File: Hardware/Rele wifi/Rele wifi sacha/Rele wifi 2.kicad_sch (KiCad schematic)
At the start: 16 parts, among them J1 Screw_Terminal_01x02, J2 Screw_Terminal_01x03, J4 Conn_01x03_Pin, K1 G5LE-1, Q2 BC337, SW1 SW_Push, U5 PC817

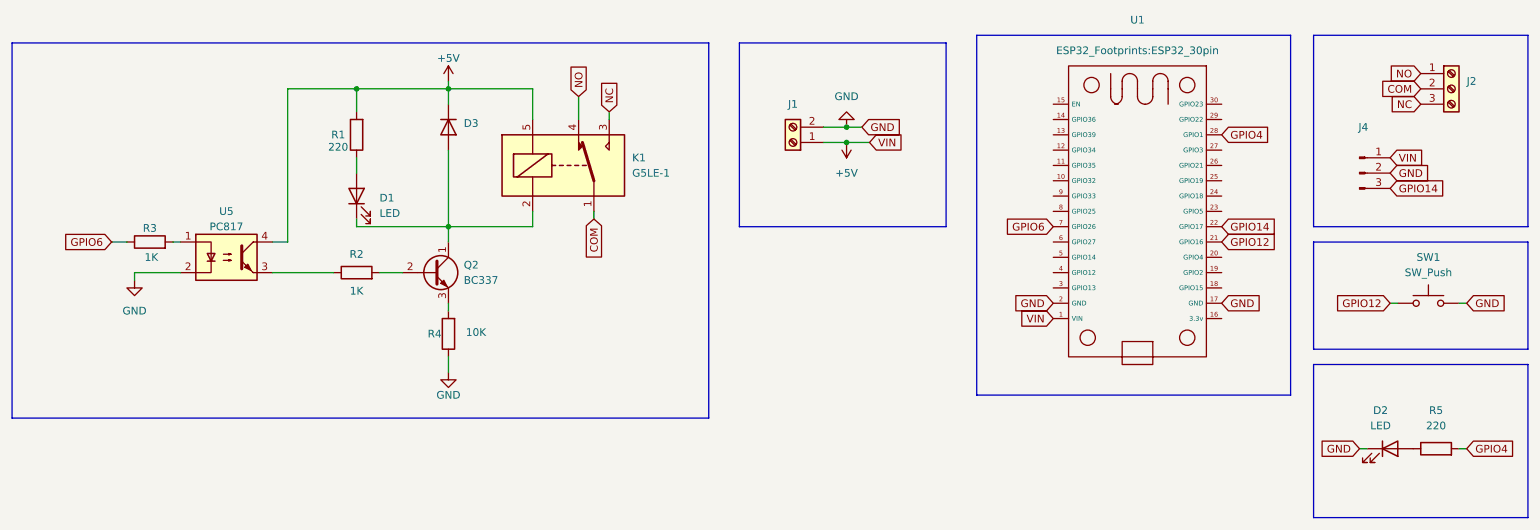
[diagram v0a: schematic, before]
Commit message: actu pcb
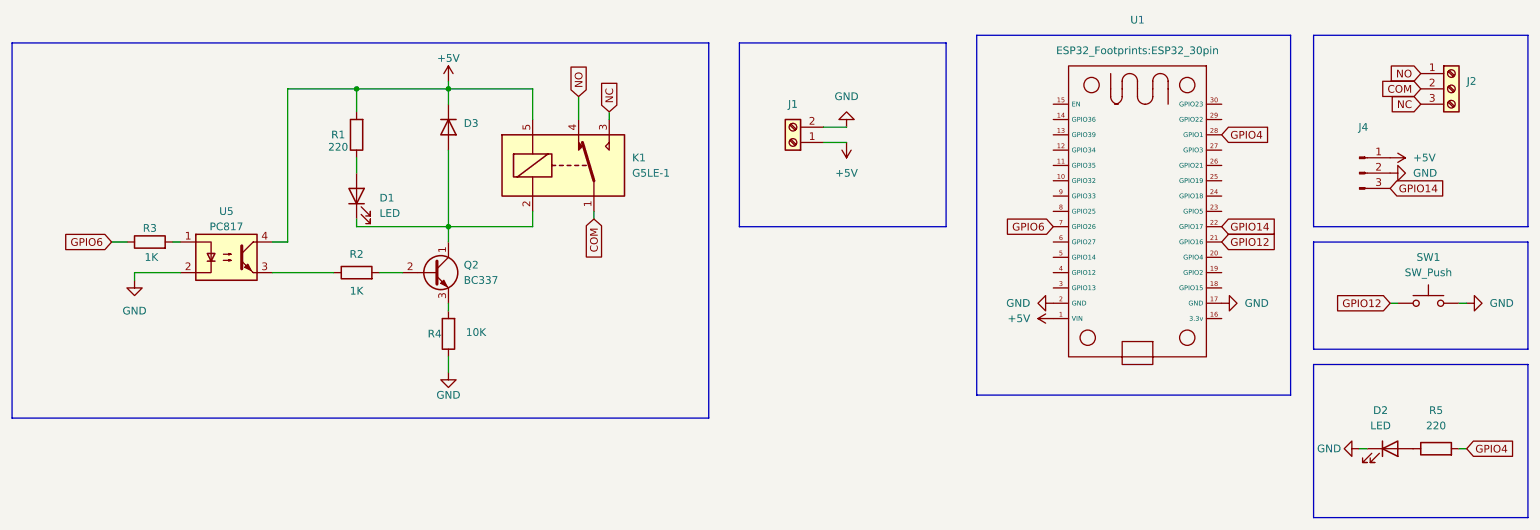
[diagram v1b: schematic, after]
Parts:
- J1: footprint TerminalBlock:TerminalBlock_MaiXu_MX126-5.0-02P_1x02_P5.00mm -> TerminalBlock_Phoenix:TerminalBlock_Phoenix_MKDS-1,5-2-5.08_1x02_P5.08mm_Horizontal
- J2: footprint TerminalBlock:TerminalBlock_MaiXu_MX126-5.0-03P_1x03_P5.00mm -> TerminalBlock_Phoenix:TerminalBlock_Phoenix_MKDS-1,5-3-5.08_1x03_P5.08mm_Horizontal
- J4: footprint Connector_PinHeader_2.00mm:PinHeader_1x03_P2.00mm_Vertical -> Connector_PinSocket_2.54mm:PinSocket_1x03_P2.54mm_Vertical

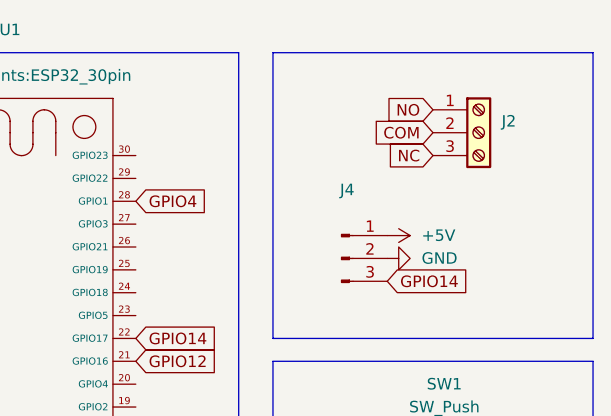
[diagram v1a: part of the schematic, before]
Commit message: actu pcb
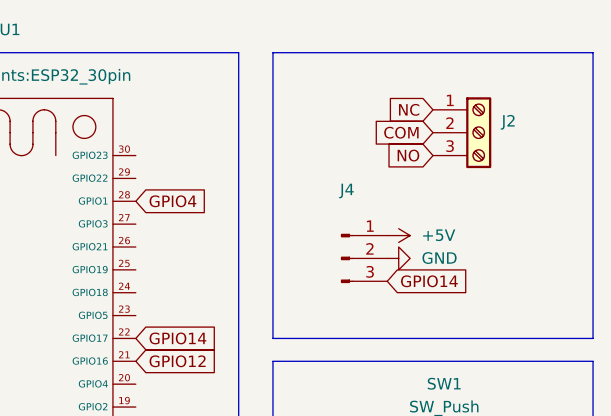
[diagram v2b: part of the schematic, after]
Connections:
- net NC: now also J2.1 (Pin_1); no longer J2.3 (Pin_3)
- net NO: now also J2.3 (Pin_3); no longer J2.1 (Pin_1)
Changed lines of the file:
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@@
 	(global_label "NO"
 		(shape input)
-		(at 264.16 21.59 180)
+		(at 264.16 26.67 180)
 		(fields_autoplaced yes)
 		(effects
@@
 		)
 		(property "Intersheetrefs" "${INTERSHEET_REFS}"
-			(at 258.5138 21.59 0)
+			(at 258.5138 26.67 0)
 			(effects
 				(font
@@
 	(global_label "NC"
 		(shape input)
-		(at 264.16 26.67 180)
+		(at 264.16 21.59 180)
 		(fields_autoplaced yes)
 		(effects
@@
 		)
 		(property "Intersheetrefs" "${INTERSHEET_REFS}"
-			(at 258.5743 26.67 0)
+			(at 258.5743 21.59 0)
 			(effects
 				(font

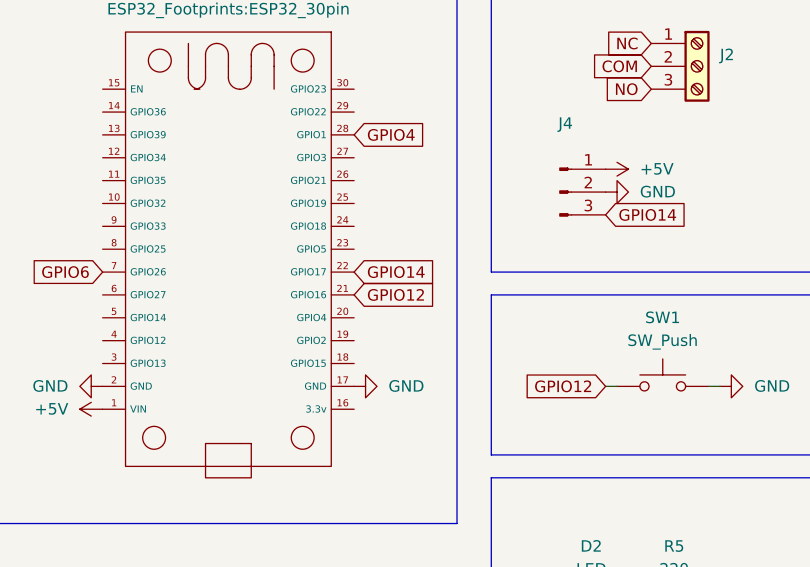
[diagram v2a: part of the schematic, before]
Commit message: actu pcb 5/10
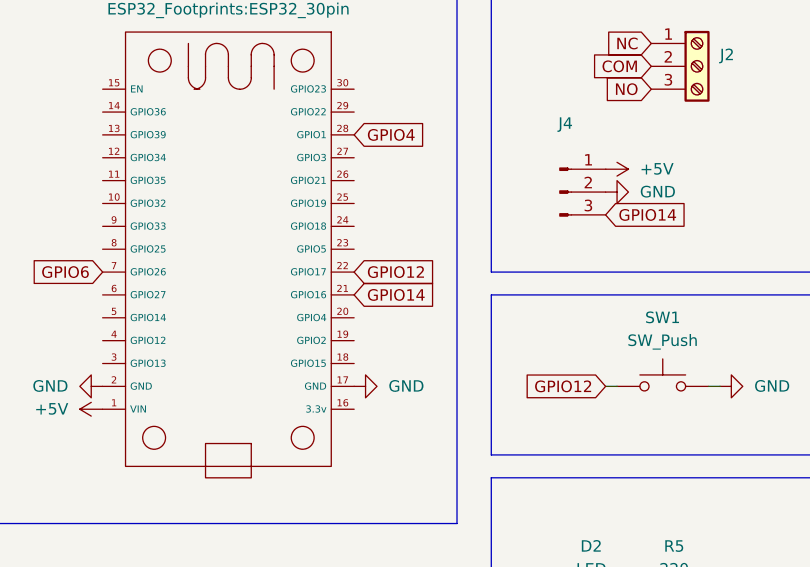
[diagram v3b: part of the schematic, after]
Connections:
- net GPIO12: now also U1.22 (GPIO17); no longer U1.21 (GPIO16)
- net GPIO14: now also U1.21 (GPIO16); no longer U1.22 (GPIO17)
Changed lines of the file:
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@@
 	(global_label "GPIO14"
 		(shape input)
-		(at 231.14 46.99 0)
+		(at 231.14 49.53 0)
 		(fields_autoplaced yes)
 		(effects
@@
 		)
 		(property "Intersheetrefs" "${INTERSHEET_REFS}"
-			(at 241.0195 46.99 0)
+			(at 241.0195 49.53 0)
 			(effects
 				(font
@@
 	(global_label "GPIO12"
 		(shape input)
-		(at 231.14 49.53 0)
+		(at 231.14 46.99 0)
 		(fields_autoplaced yes)
 		(effects
@@
 		)
 		(property "Intersheetrefs" "${INTERSHEET_REFS}"
-			(at 241.0195 49.53 0)
+			(at 241.0195 46.99 0)
 			(effects
 				(font
